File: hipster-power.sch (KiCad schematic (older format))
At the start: 14 parts, among them Q201 FDN340P, SW201 ON|OFF, U201 MCP73831, U202 XC6210A33MR-G

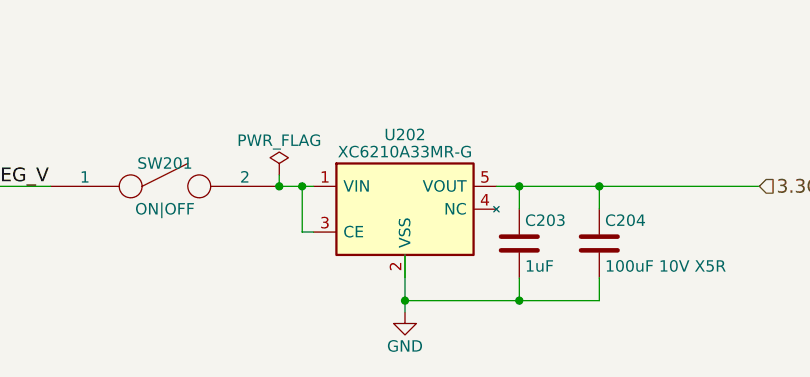
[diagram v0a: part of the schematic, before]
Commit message: Fixed some connections.  added vias
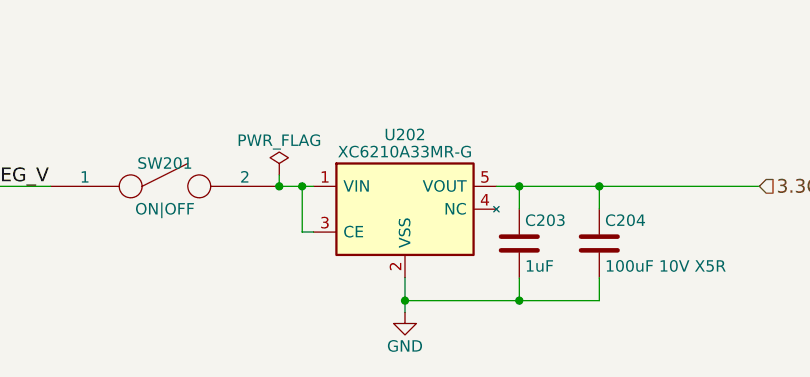
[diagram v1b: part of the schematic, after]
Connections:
- net GND: now also U202.2 (VSS)
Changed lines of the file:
@@
 Connection ~ 4400 4350
 Wire Wire Line
-	3900 4650 3900 4900
+	3900 4750 3900 4900
 Wire Wire Line
 	4400 4850 4400 4750
